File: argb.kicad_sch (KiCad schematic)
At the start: 16 parts, among them J2 Conn_01x03_MountingPin, U4 TPS22917DBV, U7 SN74LV1T125DCK

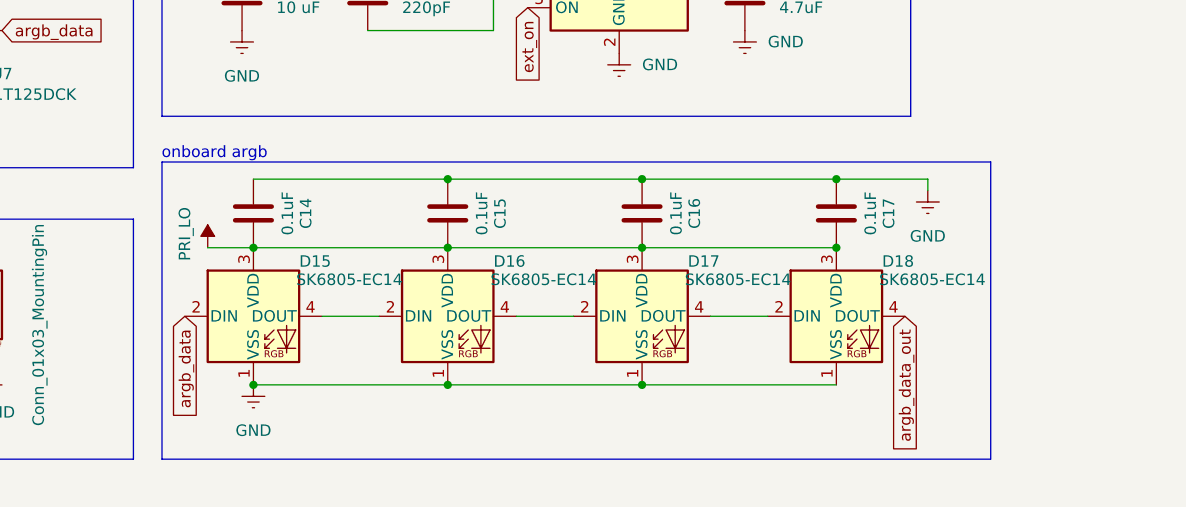
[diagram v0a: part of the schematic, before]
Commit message: final to order
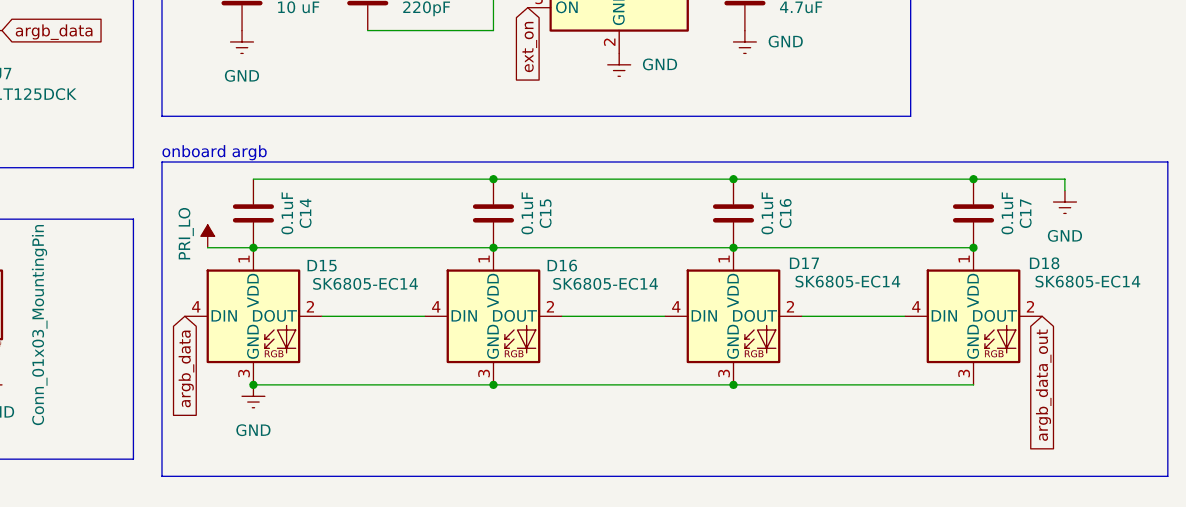
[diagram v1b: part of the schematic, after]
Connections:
- net GND: now also D15.3 (GND), D16.3 (GND), D17.3 (GND), D18.3 (GND); no longer D15.1 (VSS), D16.1 (VSS), D17.1 (VSS), D18.1 (VSS)
- net PRI_LO: now also D15.1 (VDD), D16.1 (VDD), D17.1 (VDD), D18.1 (VDD); no longer D15.3 (VDD), D16.3 (VDD), D17.3 (VDD), D18.3 (VDD)
- net argb_data: now also D15.4 (DIN); no longer D15.2 (DIN)
- net argb_data_out: now also D18.2 (DOUT); no longer D18.4 (DOUT)
- net at D17.2 (DOUT): now also D18.4 (DIN); no longer D16.4 (DOUT)
- net at D17.4 (DIN): now also D16.2 (DOUT); no longer D18.2 (DIN)
- new net: D15.2 (DOUT), D16.4 (DIN)
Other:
- moved on the sheet: C15, C16, C17, D16, D17, D18

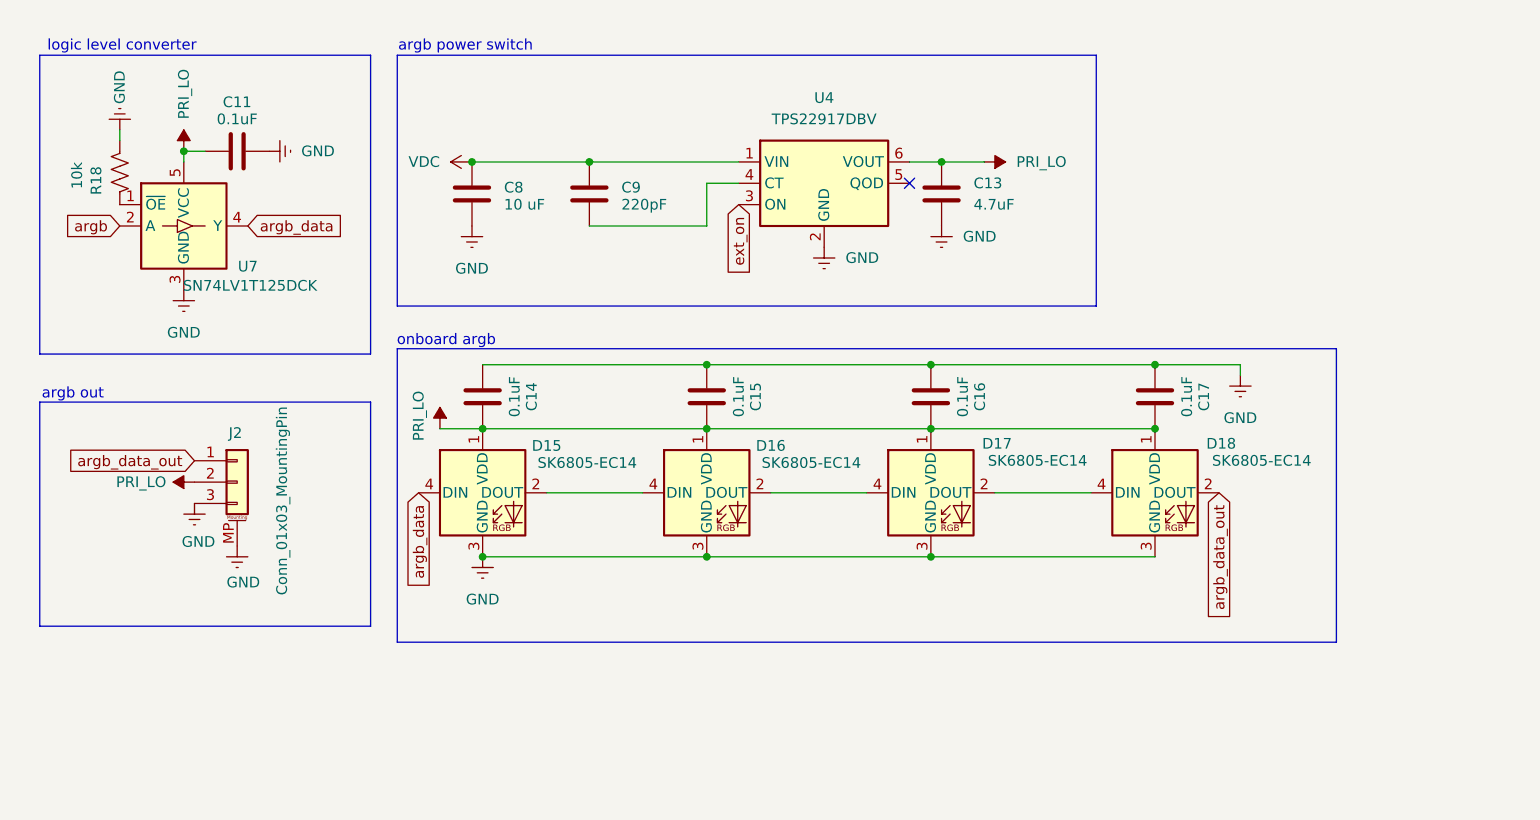
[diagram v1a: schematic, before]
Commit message: cleanup
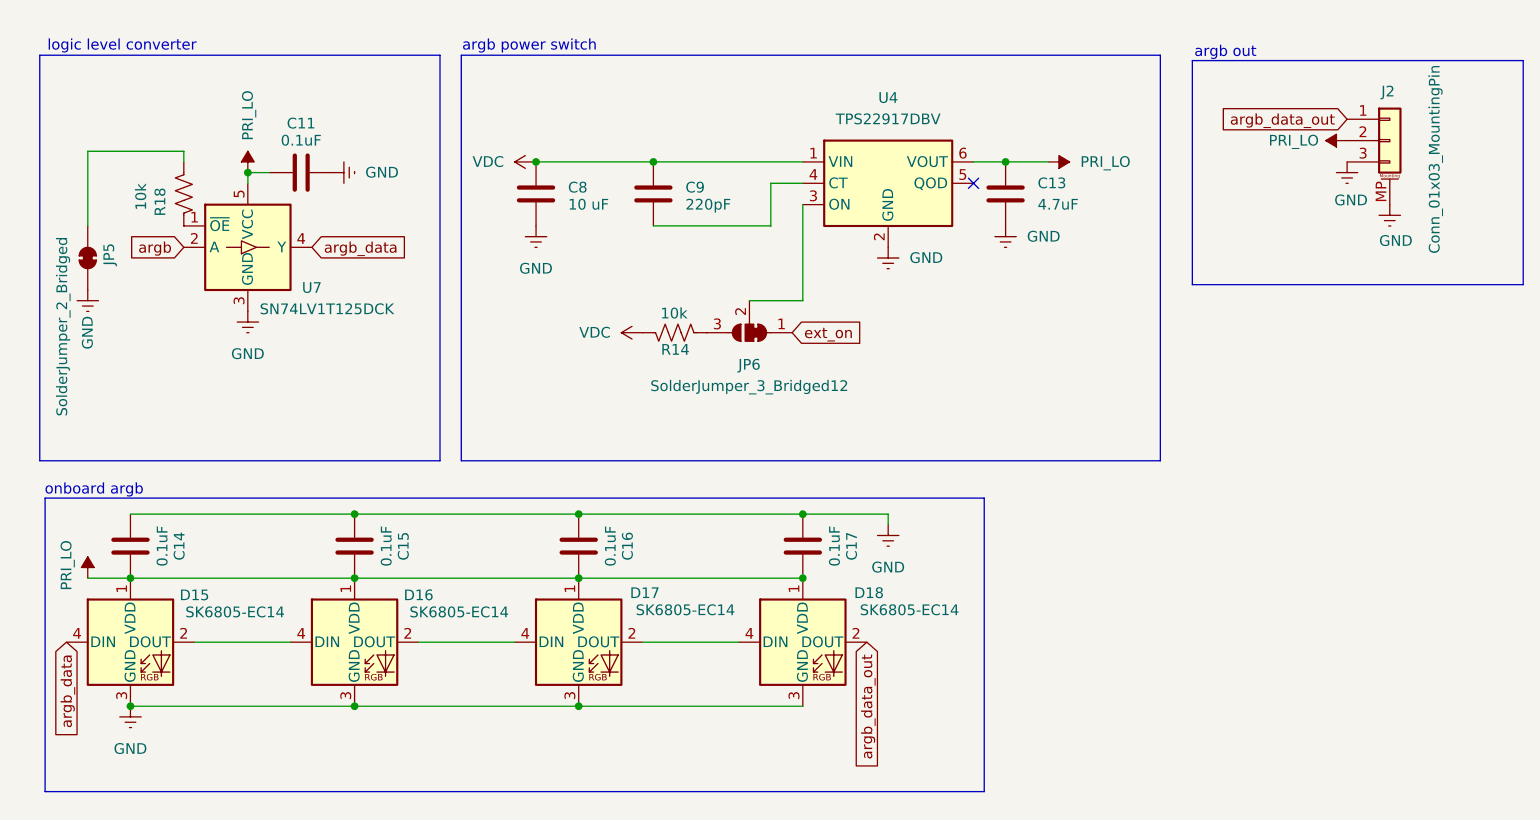
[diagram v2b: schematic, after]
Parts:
- added JP5: SolderJumper_2_Bridged, Jumper:SolderJumper-2_P1.3mm_Bridged_RoundedPad1.0x1.5mm, symbol Jumper:SolderJumper_2_Bridged
- added JP6: SolderJumper_3_Bridged12, Jumper:SolderJumper-3_P1.3mm_Bridged12_RoundedPad1.0x1.5mm, symbol Jumper:SolderJumper_3_Bridged12
- added R14: 10k, Resistor_SMD:R_0603_1608Metric, symbol Device:R_US
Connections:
- net GND: now also JP5.2 (B); no longer R18.1
- net VDC: now also R14.2
- net ext_on: now also JP6.1 (A); no longer U4.3 (ON)
- new net: JP5.1 (A), R18.1
- new net: JP6.3 (B), R14.1
- new net: JP6.2 (C), U4.3 (ON)
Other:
- moved on the sheet: C11, C13, C14, C15, C16, C17, C8, C9, D15, D16, D17, D18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
